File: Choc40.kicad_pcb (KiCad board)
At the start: 2 copper layers, 216 x 70.8 mm, 100 parts, among them SW1 SW_Push, SW10 SW_Push, SW11 SW_Push, SW12 SW_Push, SW13 SW_Push, SW14 SW_Push, SW15 SW_Push, SW16 SW_Push, SW17 SW_Push, SW18 SW_Push, SW19 SW_Push, SW2 SW_Push, SW20 SW_Push, SW21 SW_Push, SW22 SW_Push, SW23 SW_Push, SW24 SW_Push, SW25 SW_Push, SW26 SW_Push, SW27 SW_Push, SW28 SW_Push, SW29 SW_Push, SW3 SW_Push, SW30 SW_Push, SW31 SW_Push, SW32 SW_Push, SW33a1 SW_Push, SW33b1 SW_Push, SW34a1 SW_Push, SW34b1 SW_Push, SW35 SW_Push, SW36 SW_Push, SW37 SW_Push, SW38 SW_Push, SW39 SW_Push, SW4 SW_Push, SW40 SW_Push, SW5 SW_Push, SW6 SW_Push, SW7 SW_Push, SW8 SW_Push, SW9 SW_Push, SW99 SW_Push, U1 ATmega32U2-MU, Y1 Resonator_Small

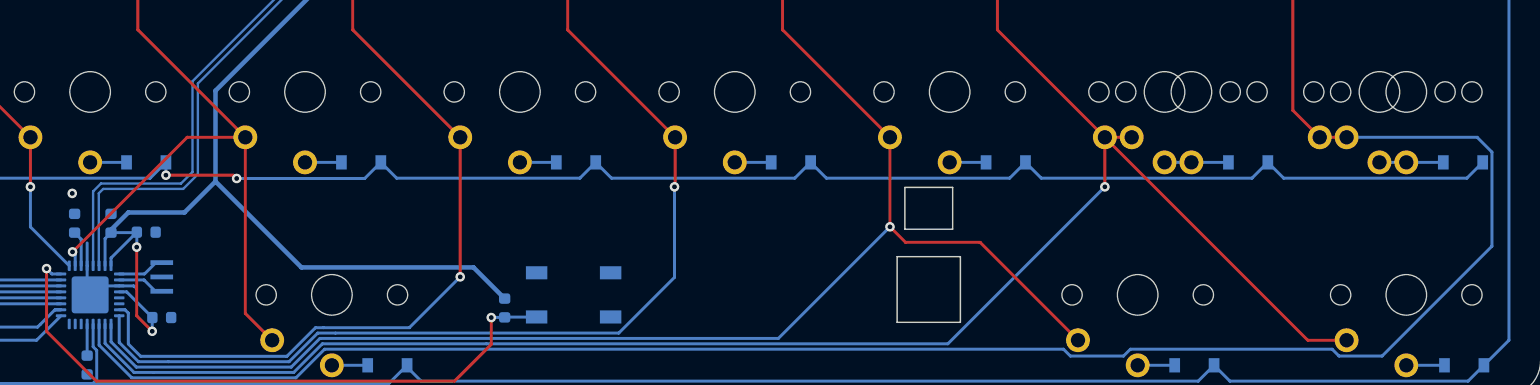
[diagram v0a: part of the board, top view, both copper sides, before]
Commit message: Production files added
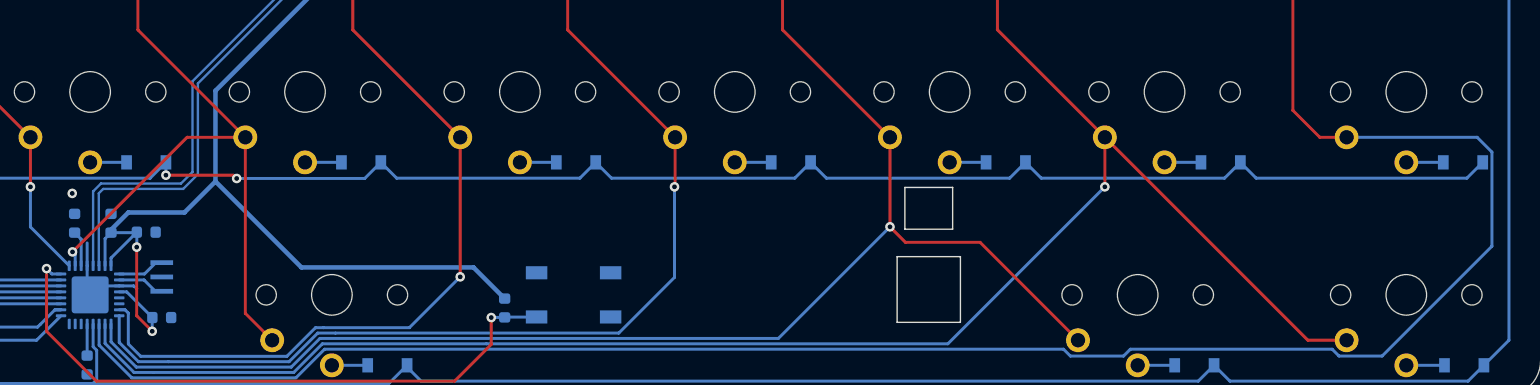
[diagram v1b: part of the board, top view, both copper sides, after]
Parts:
- removed SW33b1: SW_Push, mbk:Choc-1.25u-solder
- removed SW34b1: SW_Push, mbk:Choc-1u-solder
- moved D33 2.30 mm to (214.2, 73.4)
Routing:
- net Net-(D33-Pad2): track 5.35 -> 3.05 mm
- net col9: track 166.1 -> 163.9 mm
- net Net-(D34-Pad2): track 5.35 -> 3.10 mm
